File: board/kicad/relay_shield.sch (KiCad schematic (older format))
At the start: 13 parts

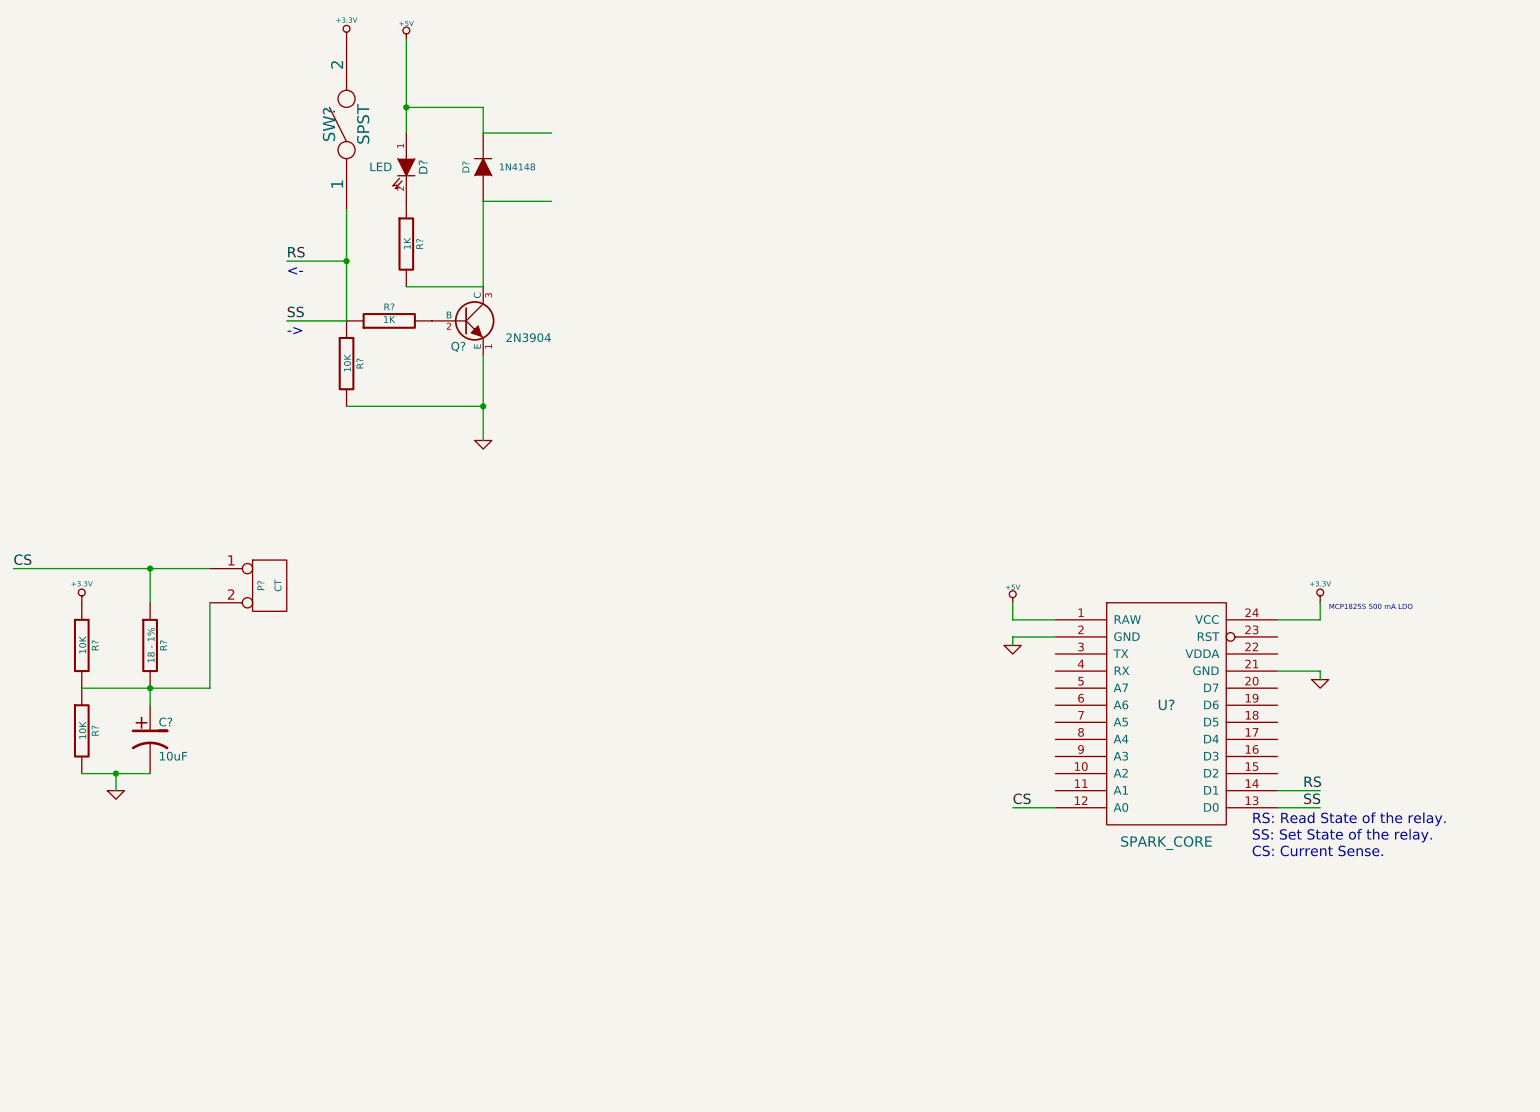
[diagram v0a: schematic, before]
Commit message: Finished schematic version 0.1.
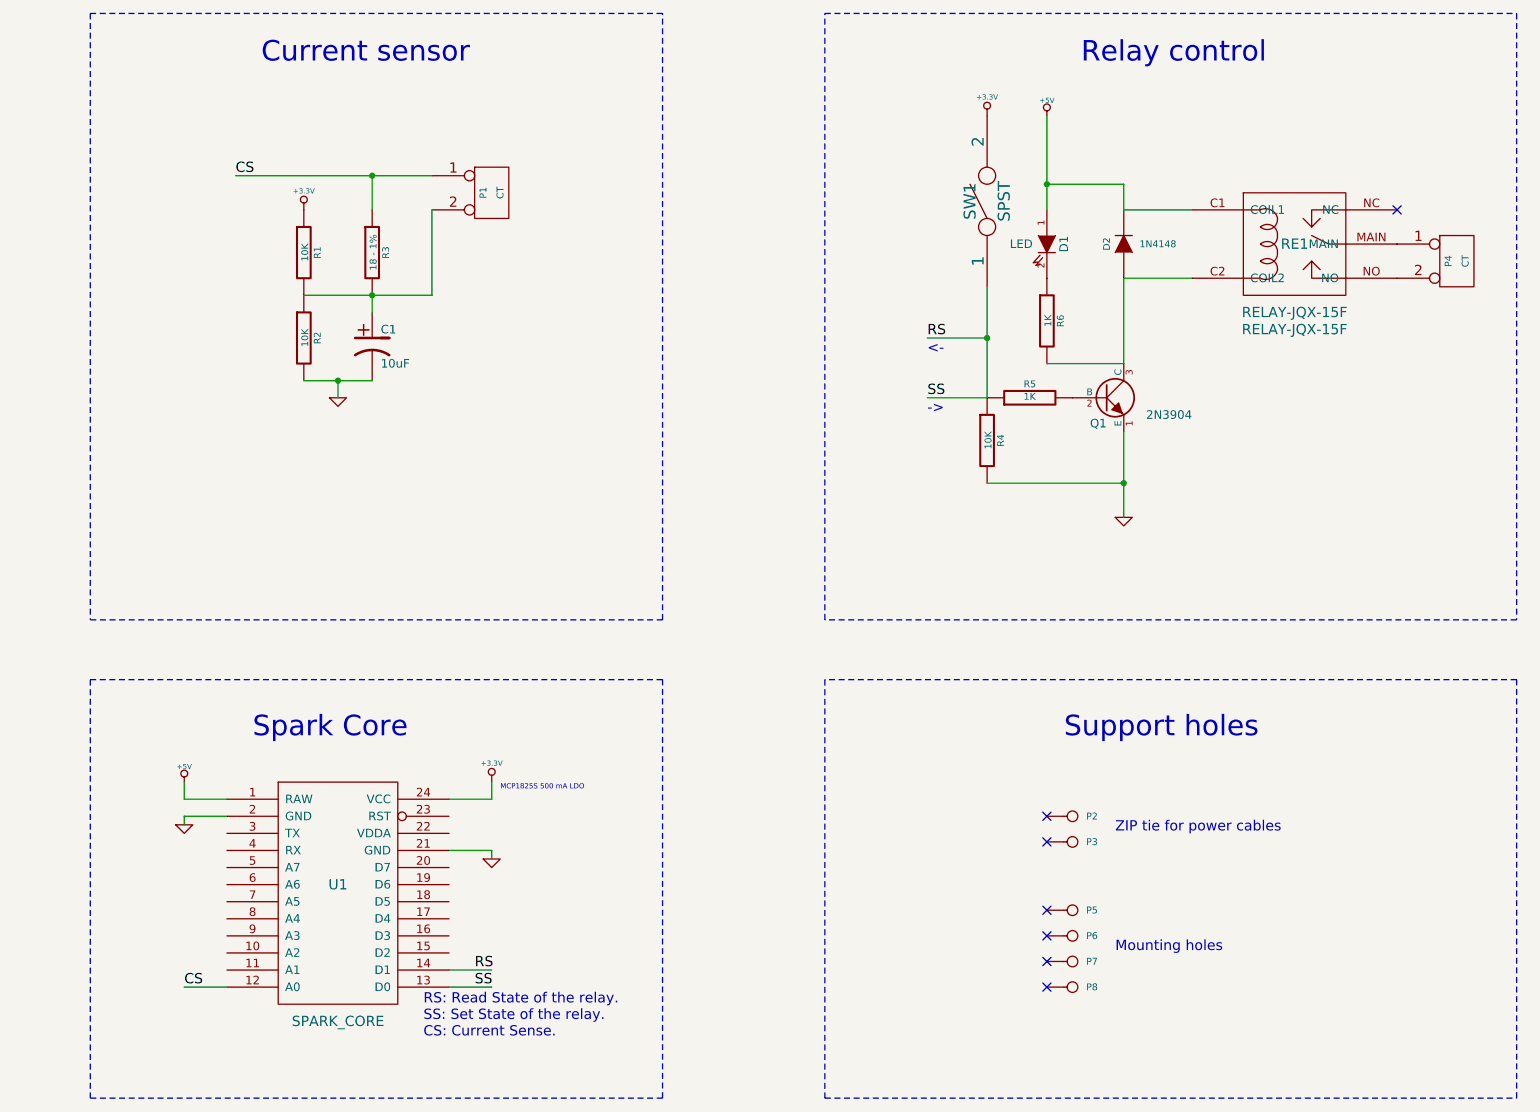
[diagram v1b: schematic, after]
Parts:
- added P2, P3, P5, P6, P7, P8: CONN_1, symbol CONN_1
- added P4: CT, symbol CONN_2
- added RE1: RELAY-JQX-15F, RELAY-JQX-15F, symbol RELAY-JQX-15F
- gave numbers to parts that had none: 13
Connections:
- no-connect marks 0 -> 7
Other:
- note added: "Current sensor"
- note added: "Mounting holes"
- note added: "Relay control"
- note added: "Spark Core"
- note added: "Support holes"
- note added: "ZIP tie for power cables"
- moved on the sheet: C1, D1, D2, P1, Q1, R1, R2, R3, R4, R5, R6, SW1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
